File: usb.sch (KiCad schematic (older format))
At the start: 1 part

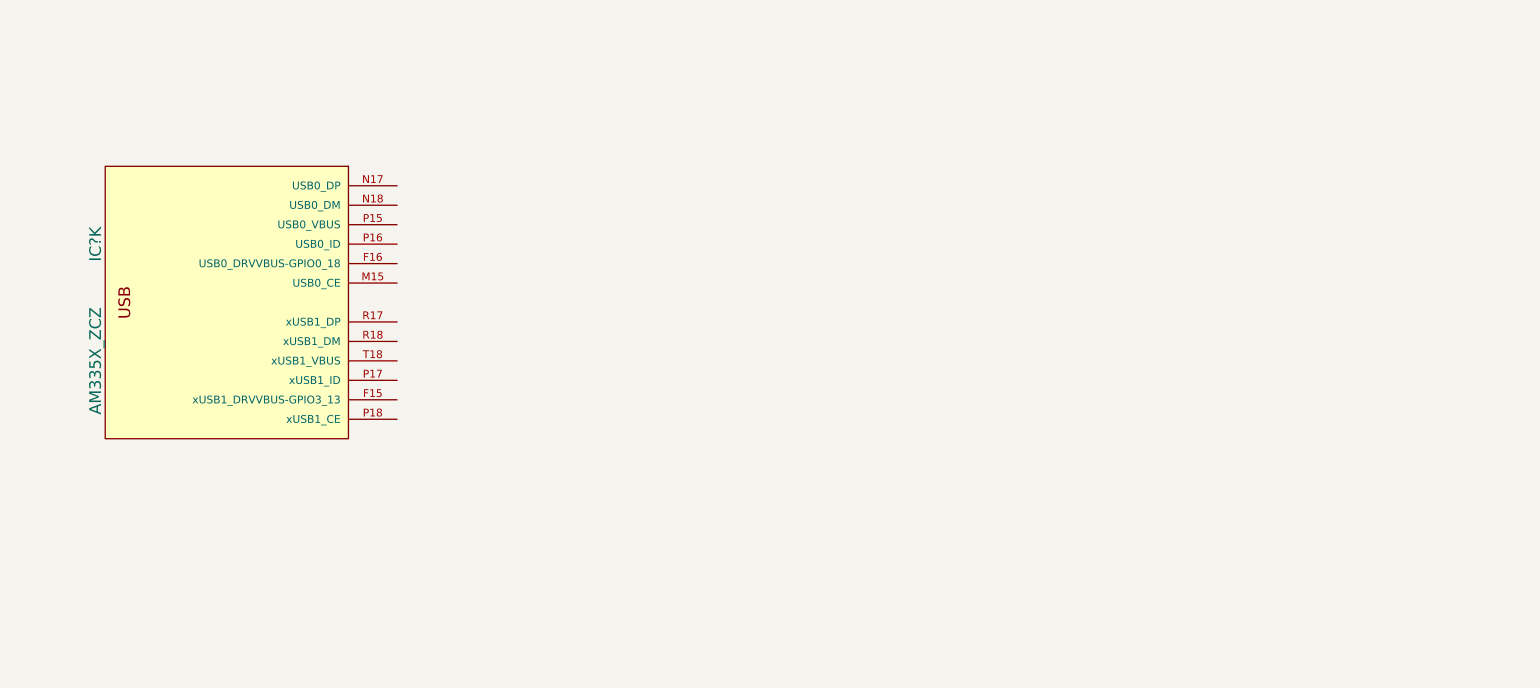
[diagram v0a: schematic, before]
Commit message: usb
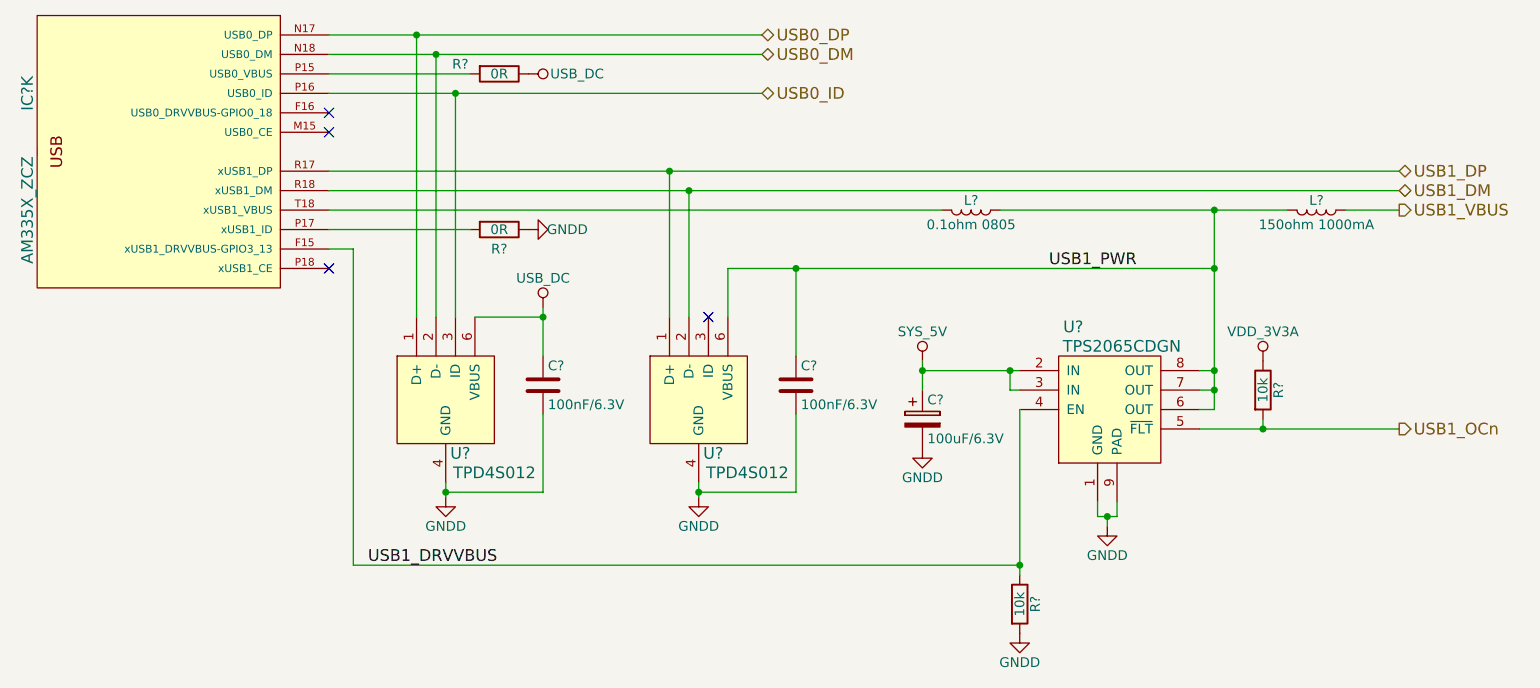
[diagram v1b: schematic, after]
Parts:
- added C? (x2): 100nF/6.3V, symbol C
- added C?: 100uF/6.3V, symbol CP
- added L?: 0.1ohm 0805, symbol L
- added L?: 150ohm 1000mA, symbol L
- added R? (x2): 0R, symbol R
- added R? (x2): 10k, symbol R
- added U? (x2): TPD4S012, symbol TPD4S012
- added U?: TPS2065CDGN, symbol TPS2065CDGN
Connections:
- net USB1_DRVVBUS: now reaches IC?.F15 (xUSB1_DRVVBUS-GPIO3_13)
- net USB1_DRVVBUS: now also R?.1, U?.4 (EN)
- net USB0_DP: now reaches IC?.N17 (USB0_DP)
- net USB0_DP: now also U?.1 (D+)
- net USB0_DM: now reaches IC?.N18 (USB0_DM)
- net USB0_DM: now also U?.2 (D-)
- net at IC?.P15 (USB0_VBUS): now also R?.2
- net USB0_ID: now reaches IC?.P16 (USB0_ID)
- net USB0_ID: now also U?.3 (ID)
- net at IC?.P17 (xUSB1_ID): now also R?.2
- net USB1_DP: now reaches IC?.R17 (xUSB1_DP)
- net USB1_DP: now also U?.1 (D+)
- net USB1_DM: now reaches IC?.R18 (xUSB1_DM)
- net USB1_DM: now also U?.2 (D-)
- net at IC?.T18 (xUSB1_VBUS): now also L?.2
- new net GNDD: C?.2, C?.2, C?.2, R?.1, R?.2, U?.1 (GND), U?.4 (GND), U?.4 (GND), U?.9 (PAD)
- new net SYS_5V: C?.1, U?.2 (IN), U?.3 (IN)
- new net USB1_OCn: R?.2, U?.5 (~FLT)
- new net USB1_PWR: C?.1, L?.1, L?.2, U?.6 (OUT), U?.6 (VBUS), U?.7 (OUT), U?.8 (OUT)
- new net USB1_VBUS: L?.1
- new net USB_DC: C?.1, R?.1, U?.6 (VBUS)
- new net VDD_3V3A: R?.1
- no-connect marks 0 -> 4
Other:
- moved on the sheet: IC?K
